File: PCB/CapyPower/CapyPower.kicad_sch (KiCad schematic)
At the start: 43 parts, among them J1 XT30PW-M, J10 XT30PW-M, J11 XT30PW-M, J12 XT30PW-M, J13 XT30PW-M, J14 XT30PW-M, J4 Conn_01x04, J8 Conn_01x02, J9 Conn_01x03

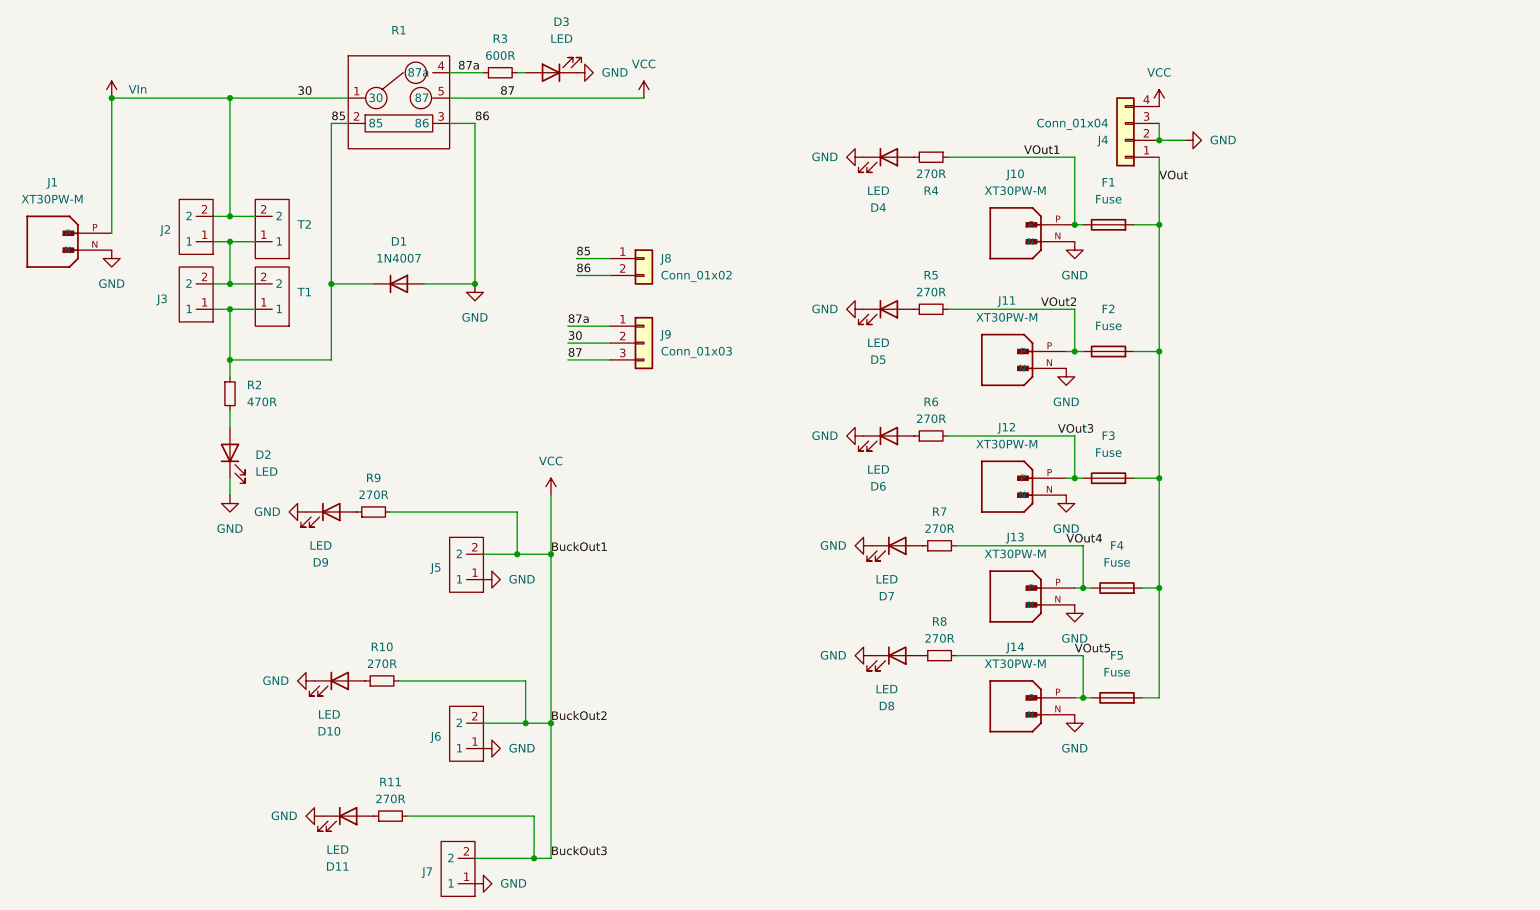
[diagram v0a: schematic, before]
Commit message: Updated CapyPower
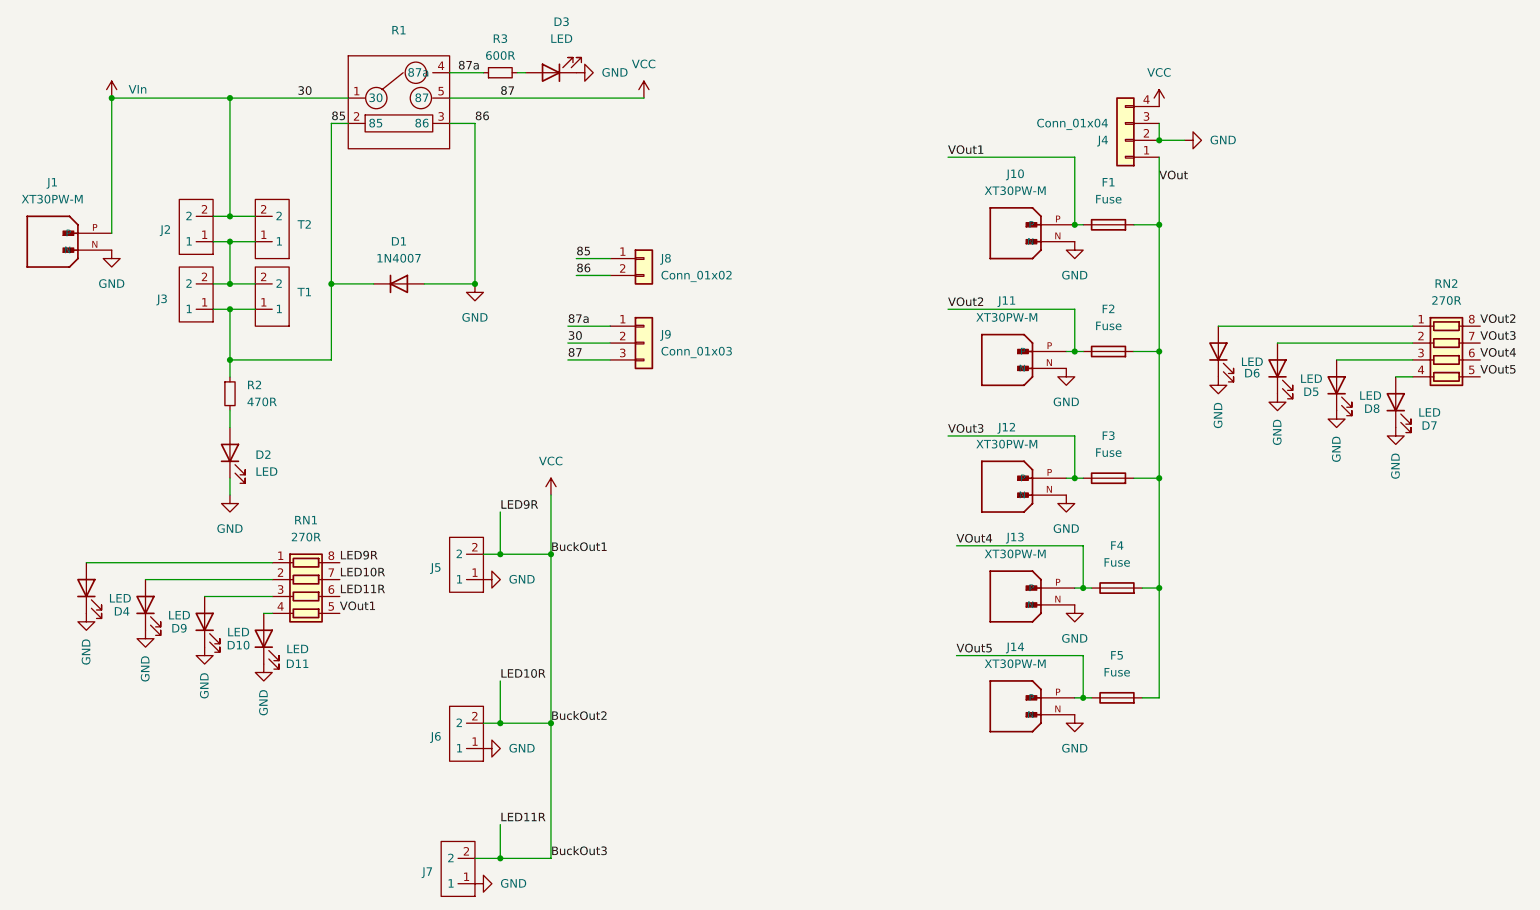
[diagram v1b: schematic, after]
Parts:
- removed R10, R11, R4, R5, R6, R7, R8, R9: 270R, Resistor_SMD:R_1206_3216Metric, symbol Device:R_Small
- added RN1, RN2: 270R, Resistor_SMD:R_Array_Convex_4x0603, symbol Device:R_Pack04
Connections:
- net VCC: now also RN1.6 (R3.2), RN1.7 (R2.2), RN1.8 (R1.2)
- net VOut1: now also RN1.5 (R4.2)
- net VOut2: now also RN2.8 (R1.2)
- net VOut3: now also RN2.7 (R2.2)
- net VOut4: now also RN2.6 (R3.2)
- net VOut5: now also RN2.5 (R4.2)
- net at D9.2 (A): now also RN1.2 (R2.1)
- net at D7.2 (A): now also RN2.4 (R4.1)
- net at D8.2 (A): now also RN2.3 (R3.1)
- net at D10.2 (A): now also RN1.3 (R3.1)
- net at D11.2 (A): now also RN1.4 (R4.1)
- net at D6.2 (A): now also RN2.1 (R1.1)
- net at D5.2 (A): now also RN2.2 (R2.1)
- net at D4.2 (A): now also RN1.1 (R1.1)
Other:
- moved on the sheet: D10, D11, D4, D5, D6, D7, D8, D9
